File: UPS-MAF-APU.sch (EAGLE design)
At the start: 35 parts, among them J1 CONNECTOR_PI_40_PIN, J2 Barrel DC In, J3 OLED, J4 OSTOQ045451, J5 External DS18B20 Temp, J6 FTDI Serial Console, J7 MagJack, U1 OLED_I2C, U2 SI7006-A20-IM, U4 INA260AIPW, U6 ENC28J60_SS, U7 5V SMPS, Y1 ECS-250-20-3X-EN-TR

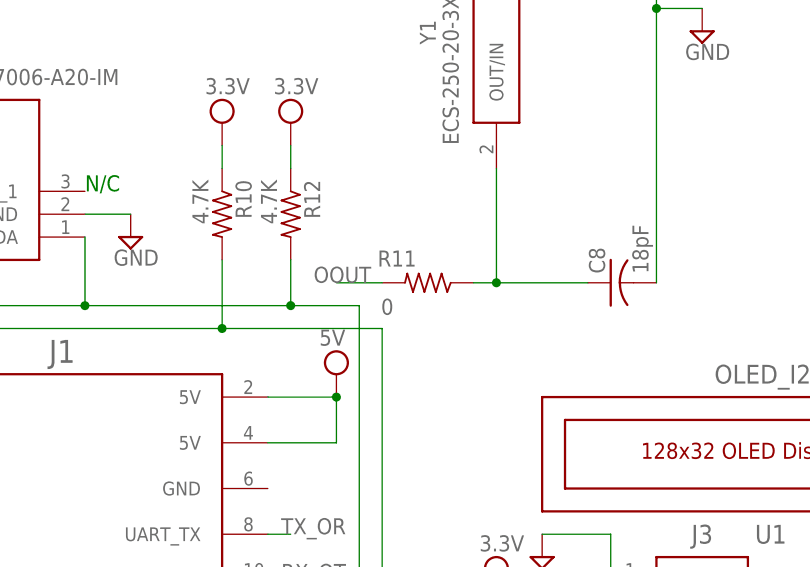
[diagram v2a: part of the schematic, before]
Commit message: README
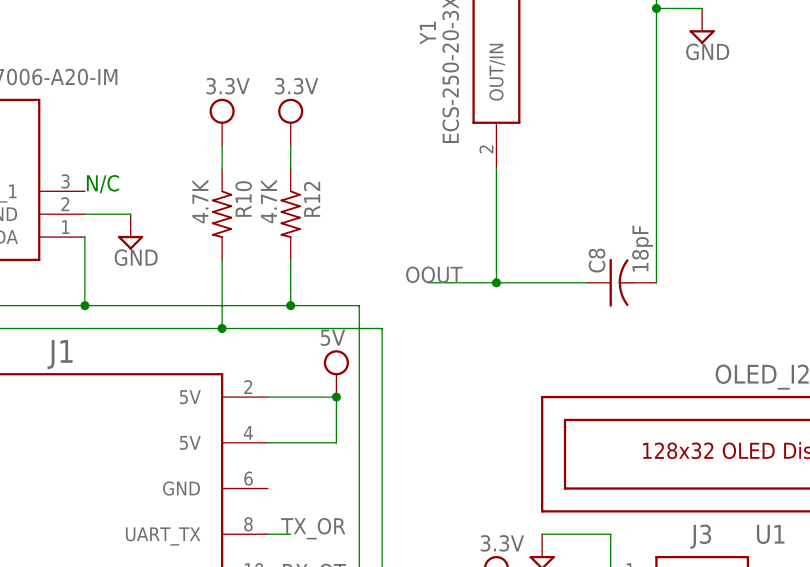
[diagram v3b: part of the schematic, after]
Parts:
- removed R11: 0, adafruit:R-US_R0805
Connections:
- removed net N$2: C8.1, R11.1, Y1.OUT/IN
- net OOUT: now also C8.1, Y1.OUT/IN; no longer R11.2
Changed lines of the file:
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@@
 <clearance class="3" value="0.254"/>
+</class>
+<class number="4" name="supply" width="0.3302" drill="0">
 </class>
 </classes>
@@
 </part>
 <part name="SYMBOL14" library="APU_ENGR480_UPS_EAGLE_Library" deviceset="3.3V" device=""/>
-<part name="R11" library="adafruit" library_urn="urn:adsk.eagle:library:420" deviceset="R-US_" device="R0805" package3d_urn="urn:adsk.eagle:package:6240566/1" value="0"/>
 <part name="R10" library="adafruit" library_urn="urn:adsk.eagle:library:420" deviceset="R-US_" device="R0805" package3d_urn="urn:adsk.eagle:package:6240566/1" value="4.7K">
 <attribute name="CRCW060350R0FKEA" value="50"/>
@@
 <attribute name="VALUE" x="109.855" y="188.595" size="1.778" layer="96"/>
 </instance>
-<instance part="R11" gate="G$1" x="193.04" y="182.88" smashed="yes" rot="R180">
-<attribute name="NAME" x="191.77" y="186.4614" size="1.778" layer="95" rot="R180"/>
-<attribute name="VALUE" x="189.23" y="181.102" size="1.778" layer="96" rot="R180"/>
-</instance>
 <instance part="R10" gate="G$1" x="170.18" y="190.5" smashed="yes" rot="R270">
 <attribute name="NAME" x="171.6786" y="194.31" size="1.778" layer="95" rot="R270"/>
@@
 </segment>
 </net>
-<net name="3.3V" class="0">
+<net name="3.3V" class="4">
 <segment>
 <pinref part="U6" gate="G$1" pin="VDDOSC"/>
@@
 </segment>
 <segment>
-<pinref part="R11" gate="G$1" pin="2"/>
-<wire x1="187.96" y1="182.88" x2="182.88" y2="182.88" width="0.1524" layer="91"/>
-<label x="180.34" y="182.88" size="1.778" layer="95"/>
+<label x="190.5" y="182.88" size="1.778" layer="95"/>
+<pinref part="C8" gate="G$1" pin="1"/>
+<wire x1="210.82" y1="182.88" x2="200.66" y2="182.88" width="0.1524" layer="91"/>
+<pinref part="Y1" gate="G$1" pin="OUT/IN"/>
+<wire x1="200.66" y1="195.58" x2="200.66" y2="182.88" width="0.1524" layer="91"/>
+<junction x="200.66" y="182.88"/>
+<wire x1="193.04" y1="182.88" x2="200.66" y2="182.88" width="0.1524" layer="91"/>
 </segment>
 </net>
@@
 </segment>
 </net>
-<net name="N$2" class="0">
-<segment>
-<pinref part="C8" gate="G$1" pin="1"/>
-<wire x1="210.82" y1="182.88" x2="200.66" y2="182.88" width="0.1524" layer="91"/>
-<pinref part="R11" gate="G$1" pin="1"/>
-<pinref part="Y1" gate="G$1" pin="OUT/IN"/>
-<wire x1="200.66" y1="182.88" x2="198.12" y2="182.88" width="0.1524" layer="91"/>
-<wire x1="200.66" y1="195.58" x2="200.66" y2="182.88" width="0.1524" layer="91"/>
-<junction x="200.66" y="182.88"/>
-</segment>
-</net>
